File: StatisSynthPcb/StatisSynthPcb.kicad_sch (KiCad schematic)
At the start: 15 parts, among them J1 Conn_01x02_Pin, J2 AudioJack3_SwitchT, SW1 SW_Push, SW2 SW_Push, U1 AP2112K-3.3, U2 PCM5102A, U3 MAX98357A

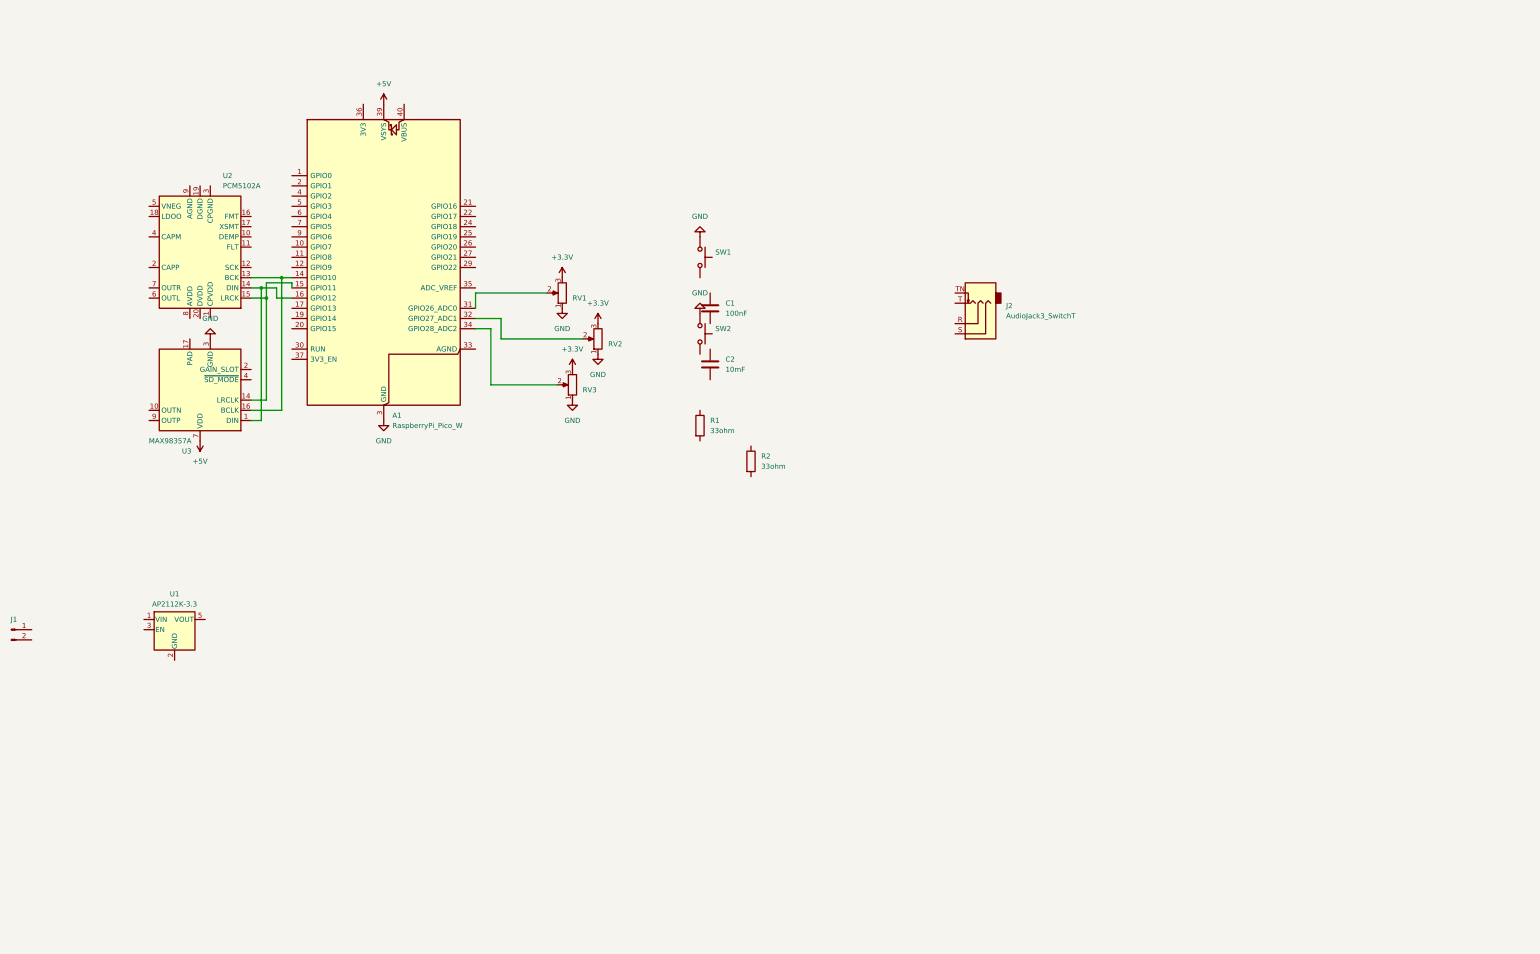
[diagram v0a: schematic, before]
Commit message: change in schematic
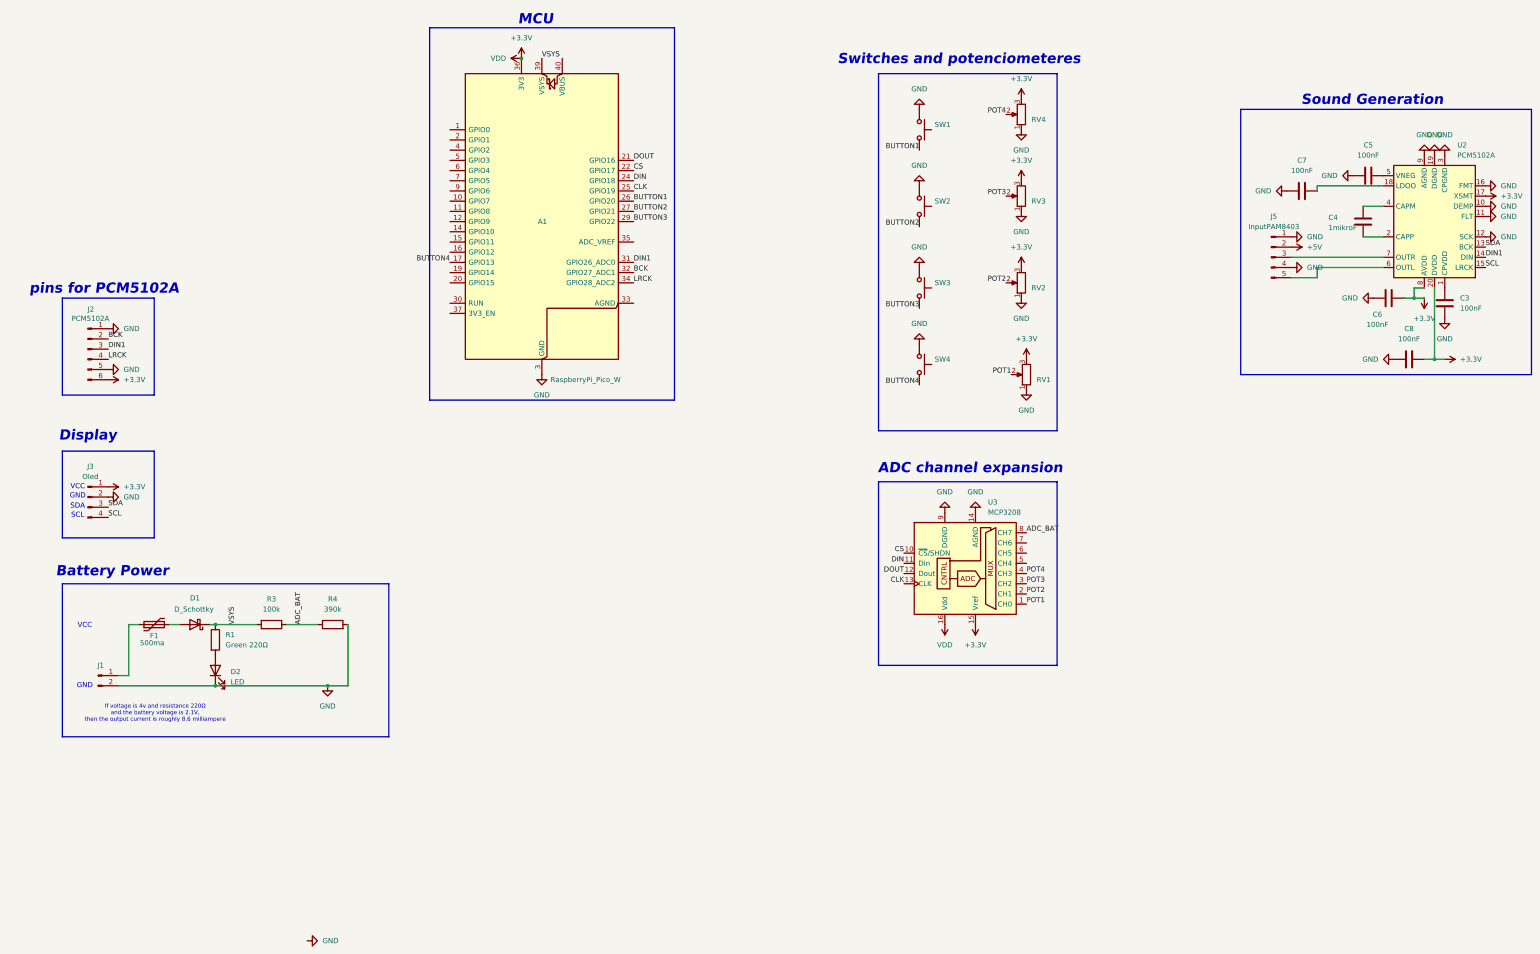
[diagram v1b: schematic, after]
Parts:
- removed C1: 100nF, Capacitor_SMD:C_0402_1005Metric_Pad0.74x0.62mm_HandSolder, symbol Device:C
- removed C2: 10mF, Capacitor_SMD:C_0805_2012Metric_Pad1.18x1.45mm_HandSolder, symbol Device:C
- removed J2: AudioJack3_SwitchT, Connector_Audio:Jack_3.5mm_CUI_SJ-3523-SMT_Horizontal, symbol Connector_Audio:AudioJack3_SwitchT
- removed R2: 33ohm, Resistor_SMD:R_0402, symbol Device:R
- removed U1: AP2112K-3.3, Package_TO_SOT_SMD:SOT-23-5_HandSoldering, symbol Regulator_Linear:AP2112K-3.3
- removed U3: MAX98357A, Package_DFN_QFN:TQFN-16-1EP_3x3mm_P0.5mm_EP1.23x1.23mm, symbol Audio:MAX98357A
- added C3, C5, C6, C7, C8: 100nF, Capacitor_SMD:C_0805_2012Metric_Pad1.18x1.45mm_HandSolder, symbol Device:C
- added C4: 1mikroF, Capacitor_SMD:C_0805_2012Metric_Pad1.18x1.45mm_HandSolder, symbol Device:C
- added D1: D_Schottky, Diode_SMD:D_SOD-123, symbol Device:D_Schottky
- added D2: LED, symbol Device:LED
- added F1: 500ma, Fuse:Fuse_1812_4532Metric_Pad1.30x3.40mm_HandSolder, symbol Device:Polyfuse
- added J2: PCM5102A, symbol Connector:Conn_01x06_Pin
- added J3: Oled, Connector_PinSocket_2.54mm:PinSocket_1x04_P2.54mm_Vertical, symbol Connector:Conn_01x04_Pin
- added J5: InputPAM8403, symbol Connector:Conn_01x05_Pin
- added R3: 100k, Resistor_THT:R_Axial_DIN0207_L6.3mm_D2.5mm_P7.62mm_Horizontal, symbol Device:R
- added R4: 390k, Resistor_THT:R_Axial_DIN0207_L6.3mm_D2.5mm_P7.62mm_Horizontal, symbol Device:R
- added RV4: R_Potentiometer, Potentiometer_THT:Potentiometer_Alps_RK09K_Single_Vertical, symbol Device:R_Potentiometer
- added SW3, SW4: SW_Push, Button_Switch_THT:SW_PUSH_6mm, symbol Switch:SW_Push
- added U3: MCP3208, Package_DIP:DIP-16_W7.62mm_Socket_LongPads, symbol Analog_ADC:MCP3208
- R1: value 33ohm -> Green 220Ω; footprint Resistor_SMD:R_0402 -> (none)
- RV1, RV2, RV3: footprint (none) -> Potentiometer_THT:Potentiometer_Alps_RK09K_Single_Vertical
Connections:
- net +3.3V: now also A1.36 (3V3), U2.17 (XSMT), U2.20 (DVDD), U2.8 (AVDD), C6.2, C8.2, J2.6 (Pin_6), J3.1 (Pin_1), RV4.3, U3.15 (Vref), U3.16 (Vdd)
- net +5V: now also J5.2 (Pin_2); no longer A1.39 (VSYS)
- net GND: now also J1.2 (Pin_2), U2.10 (DEMP), U2.11 (FLT), U2.12 (SCK), U2.16 (FMT), U2.19 (DGND), U2.3 (CPGND), U2.9 (AGND), C3.2, C5.1, C6.1, C7.1, C8.1, D2.1 (K), J2.1 (Pin_1), J2.5 (Pin_5), J3.2 (Pin_2), J5.1 (Pin_1), J5.4 (Pin_4), R4.2, RV4.1, SW3.1, SW4.1, U3.14 (AGND), U3.9 (DGND)
- net BUTTON1: now reaches SW1.2
- net BUTTON1: now also A1.26 (GPIO20)
- net at U2.1 (CPVDD): now also C3.1
- net at A1.14 (GPIO10): no longer U2.13 (BCK)
- net at A1.16 (GPIO12): no longer U2.14 (DIN)
- net at A1.15 (GPIO11): no longer U2.15 (LRCK)
- net at U2.18 (LDOO): now also C7.2
- net at U2.2 (CAPP): now also C4.2
- net at U2.4 (CAPM): now also C4.1
- net at U2.5 (VNEG): now also C5.2
- net at U2.6 (OUTL): now also J5.5 (Pin_5)
- net at U2.7 (OUTR): now also J5.3 (Pin_3)
- net LRCK: now reaches A1.34 (GPIO28_ADC2)
- net LRCK: now also J2.4 (Pin_4); no longer RV3.2
- net DIN1: now reaches A1.31 (GPIO26_ADC0)
- net DIN1: now also U2.14 (DIN), J2.3 (Pin_3); no longer RV1.2
- net BUTTON4: now reaches A1.17 (GPIO13)
- net BUTTON4: now also SW4.2
- net DOUT: now reaches A1.21 (GPIO16)
- net DOUT: now also U3.12 (Dout)
- net CS: now reaches A1.22 (GPIO17)
- net CS: now also U3.10 (~{CS}/SHDN)
- net DIN: now reaches A1.24 (GPIO18)
- net DIN: now also U3.11 (Din)
- net CLK: now reaches A1.25 (GPIO19)
- net CLK: now also U3.13 (CLK)
- net BUTTON2: now reaches A1.27 (GPIO21)
- net BUTTON2: now also SW2.2
- net BUTTON3: now reaches A1.29 (GPIO22)
- net BUTTON3: now also SW3.2
- net BCK: now reaches A1.32 (GPIO27_ADC1)
- net BCK: now also J2.2 (Pin_2); no longer RV2.2
- net at J1.1 (Pin_1): now also F1.1
- net VSYS: now reaches R1.1
- net VSYS: now also A1.39 (VSYS), D1.1 (K), R3.2
- net at R1.2: now also D2.2 (A)
- new net: D1.2 (A), F1.2
- new net ADC_BAT: R3.1, R4.1, U3.8 (CH7)
- new net POT1: RV1.2, U3.1 (CH0)
- new net POT2: RV2.2, U3.2 (CH1)
- new net POT3: RV3.2, U3.3 (CH2)
- new net POT4: RV4.2, U3.4 (CH3)
- new net SCL: J3.4 (Pin_4), U2.15 (LRCK)
- new net SDA: J3.3 (Pin_3), U2.13 (BCK)
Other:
- note added: "ADC channel expansion"
- note added: "Battery Power"
- note added: "Display"
- note added: "GND"
- note added: "If voltage is 4v and resistance 220Ω and the battery voltage is 2.1V, then the output current is roughly 8.6 milliampere"
- note added: "MCU"
- note added: "SCL"
- note added: "SDA"
- note added: "Sound Generation"
- note added: "Switches and potenciometeres"
- note added: "VCC"
- note added: "pins for PCM5102A"
- moved on the sheet: A1, J1, RV1, RV2, RV3, SW1, SW2
